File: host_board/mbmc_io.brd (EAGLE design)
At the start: 116.5 x 81.3 mm, 71 parts, among them IC1 ULN2803, IC2 DIP Socket, IC3 REF02 5 VOLTS, IC4 5 VOLTS, IC5 12 VOLTS, IC6 3.3 VOLTS, J1 1-1586043-4, J2 1586044-4

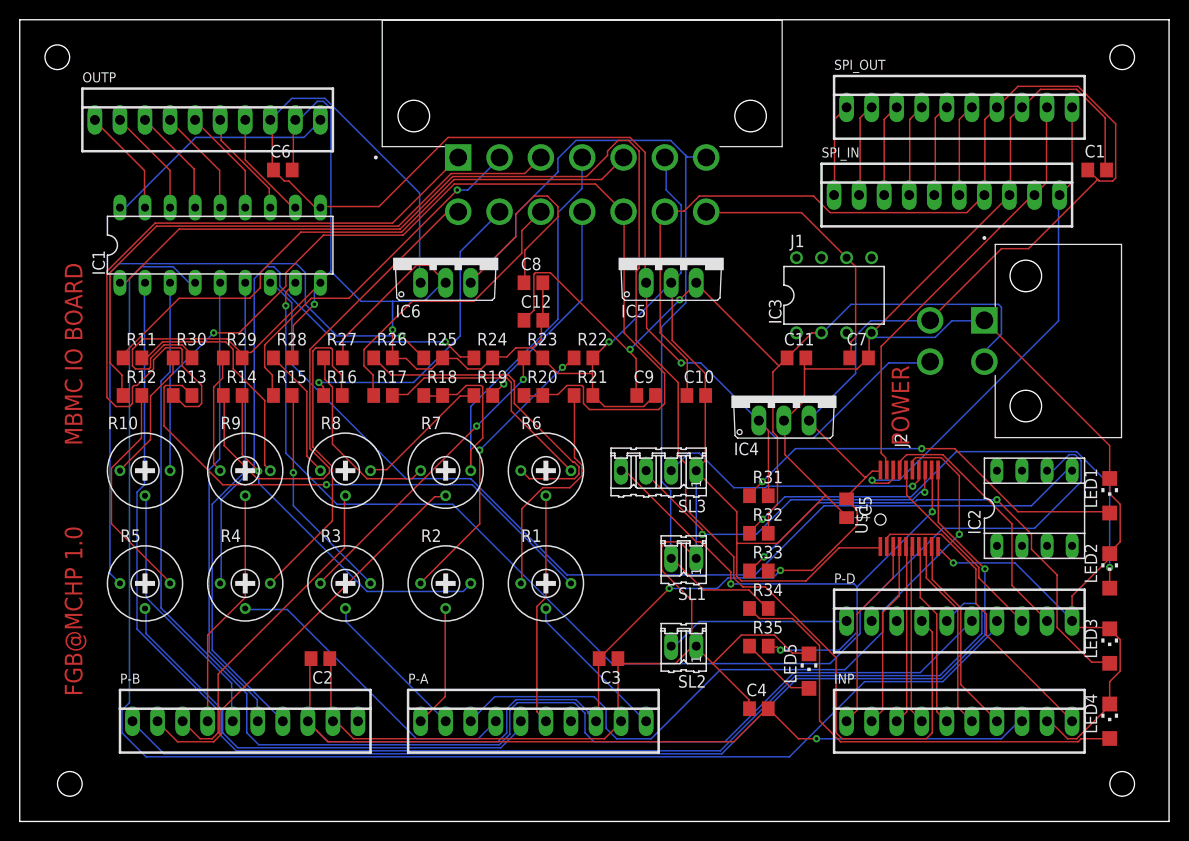
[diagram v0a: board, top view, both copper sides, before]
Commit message: up, order pcb
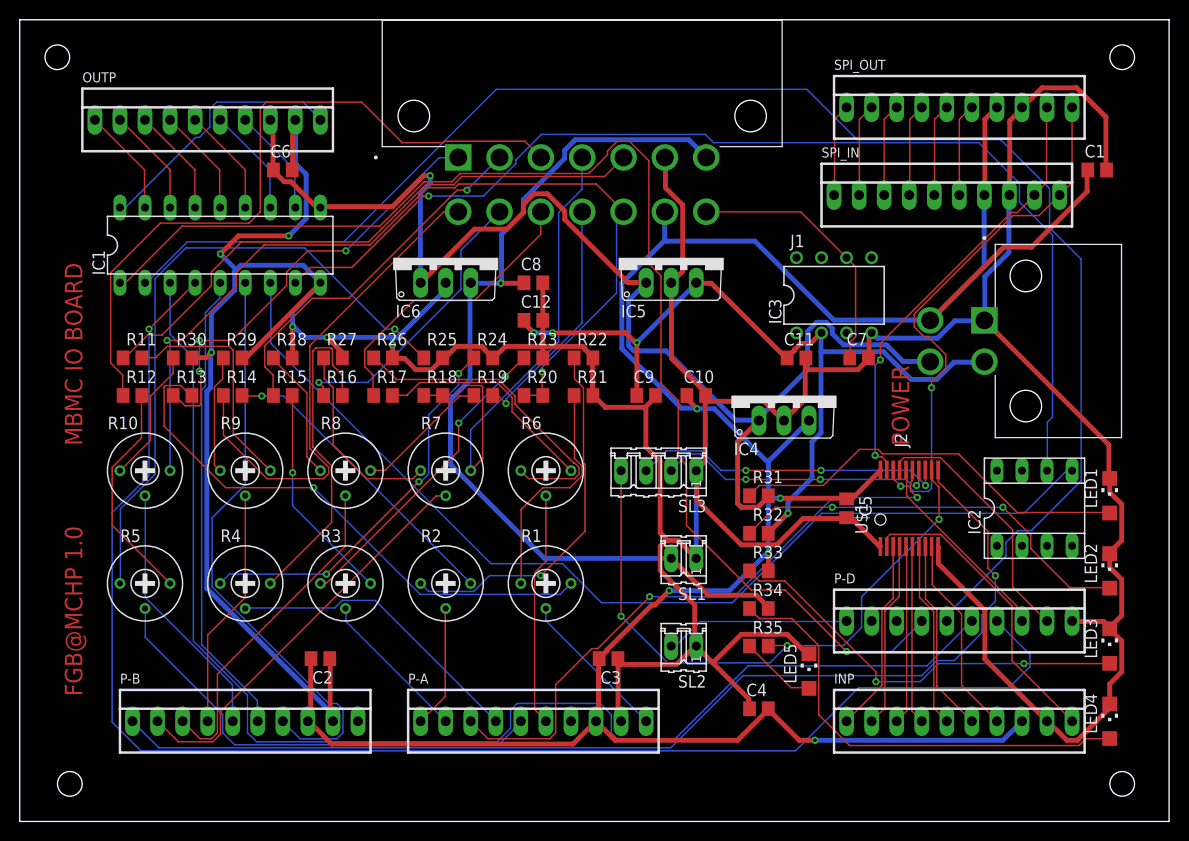
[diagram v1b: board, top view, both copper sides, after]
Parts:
- R1, R10, R2, R3, R4, R5, R6, R7, R8, R9: value (none) -> 200
- R11, R12, R15, R16, R17, R18, R19, R20: value (none) -> 9.85k
- R13, R14: value (none) -> 811
- R21, R22: value (none) -> 3820
- R23, R24, R25, R26, R27, R28, R29, R30: value (none) -> 1.28k
- R31: value (none) -> 10k
- R32: value (none) -> 5k
- R33, R34, R35: value (none) -> 1k
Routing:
- net VDD: track 302.0 -> 258.0 mm, vias 3 -> 5
- net N$74: track 75.0 -> 44.6 mm, vias 0 -> 3
- net N$31: track 150.2 -> 129.6 mm, vias 0 -> 1
- net N$14: track 59.8 -> 39.4 mm, vias 1 -> 3
- net N$32: track 139.5 -> 155.6 mm
- net +3V3: track 110.4 -> 94.8 mm, vias 0 -> 1
- net VSS: track 495.7 -> 480.5 mm, vias 4 -> 6
- net N$43: track 75.9 -> 62.2 mm, vias 1 -> 2
- net N$71: track 103.7 -> 92.2 mm, vias 1 -> 2
- net N$36: track 48.8 -> 60.1 mm
- net N$72: track 61.5 -> 72.4 mm
- net +24V: track 139.7 -> 129.1 mm
- net N$77: track 51.9 -> 41.9 mm
- net N$38: track 122.6 -> 112.7 mm
- net +12V: track 93.8 -> 84.5 mm, vias 2 -> 4
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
